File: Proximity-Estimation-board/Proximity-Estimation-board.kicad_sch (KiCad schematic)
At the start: 19 parts, among them Q1 TEFT4300, Q2 TEFT4300, U1 ArduinoNano33BLE, U2 OPA340P, U3 HC-SR04, U4 OPA340P

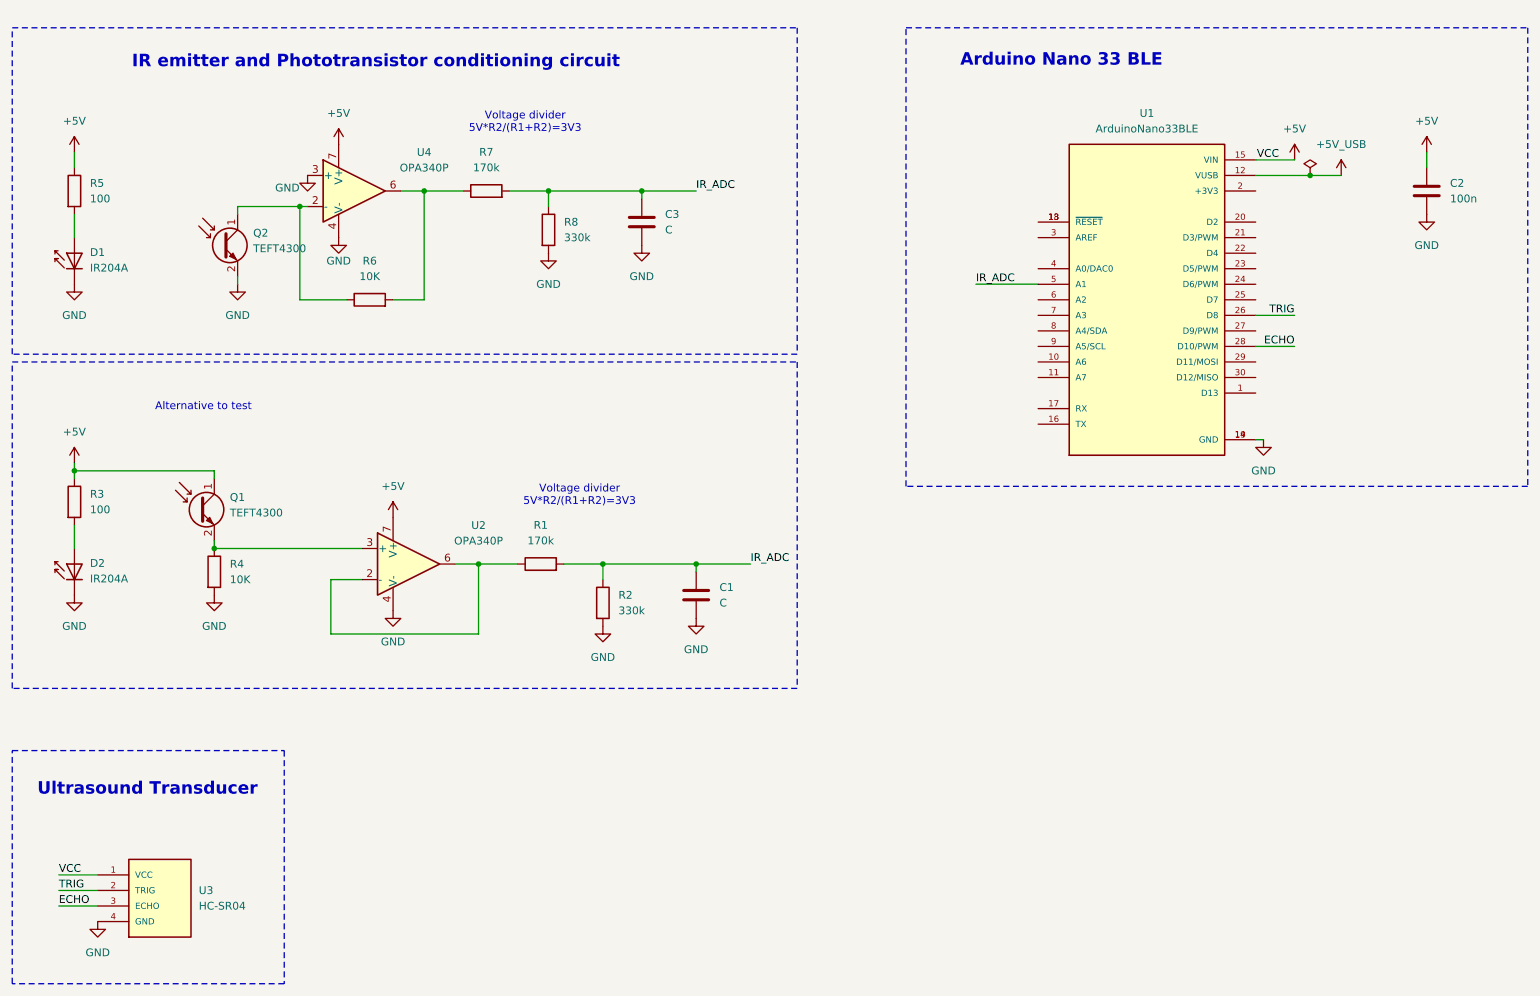
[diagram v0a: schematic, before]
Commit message: final schematic
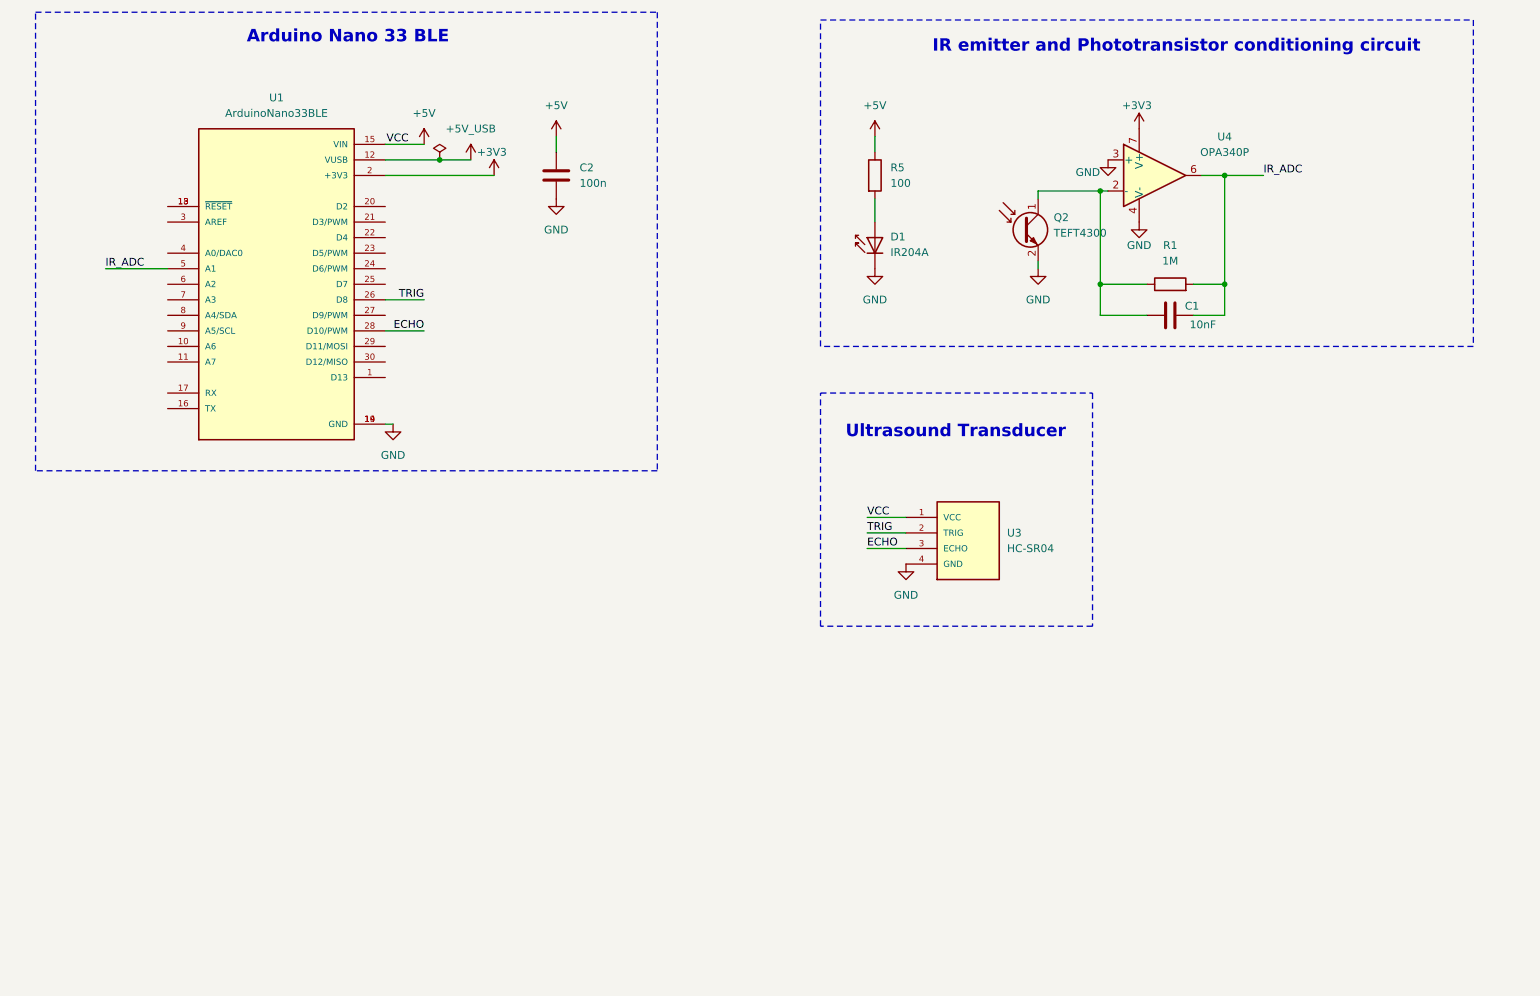
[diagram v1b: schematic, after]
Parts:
- removed C3: C, symbol Device:C
- removed D2: IR204A, LED_THT:LED_D3.0mm_IRBlack, symbol LED:IR204A
- removed Q1: TEFT4300, LED_THT:LED_D3.0mm_Clear, symbol Sensor_Optical:TEPT4400
- removed R2, R8: 330k, symbol Device:R
- removed R3: 100, symbol Device:R
- removed R4, R6: 10K, symbol Device:R
- removed R7: 170k, symbol Device:R
- removed U2: OPA340P, Package_DIP:DIP-8_W7.62mm, symbol Amplifier_Operational:OPA340P
- C1: value C -> 10nF
- R1: value 170k -> 1M
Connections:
- net +5V: no longer U4.7 (V+)
- net GND: no longer C1.2
- net IR_ADC: now also C1.2, U4.6; no longer C1.1
- net at R1.1: now also C1.1, Q2.1 (C), U4.2 (-)
- net +3V3: now reaches U1.2 (+3V3)
- net +3V3: now also U4.7 (V+)
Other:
- note removed: "Alternative to test"
- note removed: "Voltage divider 5V*R2/(R1+R2)=3V3"
- moved on the sheet: C2, D1, Q2, R5, U1, U3, U4
